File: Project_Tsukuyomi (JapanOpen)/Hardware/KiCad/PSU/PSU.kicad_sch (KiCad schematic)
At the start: 52 parts, among them J1 USB_C_Receptacle_USB2.0, J2 Conn_01x08_Socket, J3 Conn_01x08_Socket, J4 Conn_01x04_Socket, J5 Conn_01x02_Socket, J6 Conn_01x02_Socket, Q1 PMOS, SW1 SW_Push, SW2 SW_Push, U1 W25Q128JVS, U2 RP2040, U3 SFH617A-1, U4 AZ1084-5.0, Y1 Crystal_GND24

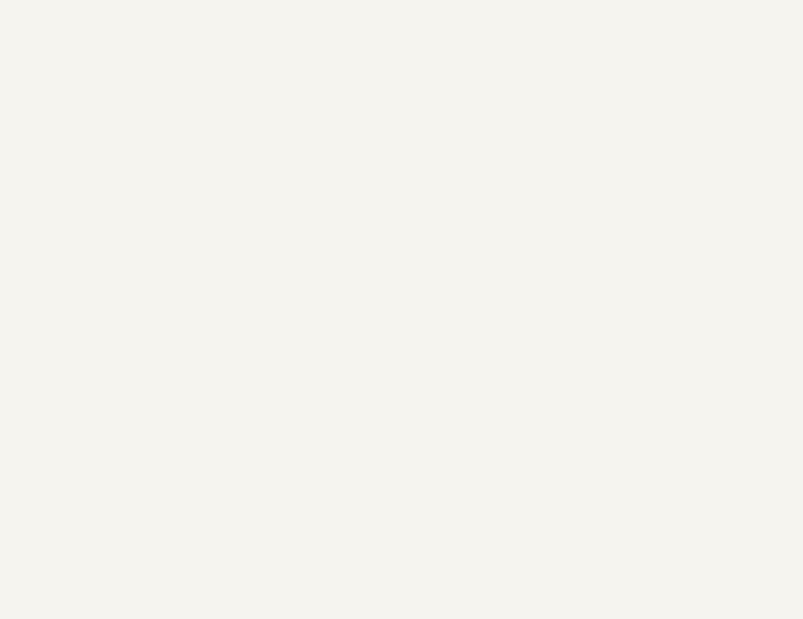
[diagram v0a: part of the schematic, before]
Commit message: KiCad変更
ごめんさい。溜めました
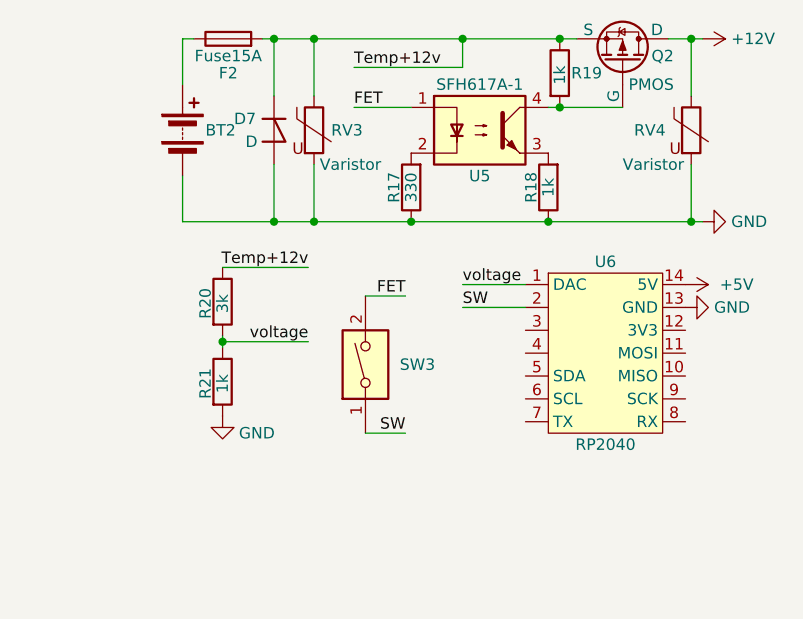
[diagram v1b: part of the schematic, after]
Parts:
- added BT2: Battery, Connector_AMASS:AMASS_XT60-M_1x02_P7.20mm_Vertical, symbol Device:Battery
- added D7: D, Diode_THT:D_DO-27_P12.70mm_Horizontal, symbol Device:D_Shockley
- added F2: Fuse15A, Fuse:Fuseholder_Clip-5x20mm_Littelfuse_520_Inline_P20.50x5.80mm_D1.30mm_Horizontal, symbol Device:Fuse
- added Q2: PMOS, Package_TO_SOT_SMD:TO-252-2, symbol Simulation_SPICE:PMOS
- added R17: 330, Resistor_SMD:R_0402_1005Metric, symbol Device:R
- added R18, R19, R21: 1k, Resistor_SMD:R_0402_1005Metric, symbol Device:R
- added R20: 3k, Resistor_SMD:R_0402_1005Metric, symbol Device:R
- added RV3, RV4: Varistor, Varistor:RV_Disc_D9mm_W3.3mm_P5mm, symbol Device:Varistor
- added SW3: SW_DIP_x01, symbol Switch:SW_DIP_x01
- added U5: SFH617A-1, Package_DIP:DIP-4_W7.62mm, symbol Isolator:SFH617A-1
- added U6: RP2040, symbol seeeduino_xiao:Seeeduino_Xiao
- C1, C11, C2, C3, C6, C7, C8, C9: LCSC (none) -> C1525
- C4, C5: LCSC (none) -> C1557
- R1, R15, R16, R2, R3, R4, R9: LCSC (none) -> C11702
- R10, R11: LCSC (none) -> C25905
- R12, R13: LCSC (none) -> C25100
- R14: LCSC (none) -> C25104
- R5: LCSC (none) -> C25076
- R8: LCSC (none) -> C25784
- U1: LCSC (none) -> C97521
- U2: LCSC (none) -> C2040
- Y1: LCSC (none) -> C7294610
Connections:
- net +12V: now also Q2.1 (D), RV4.1
- net FET: now also SW3.2, U5.1
- net GND: now also BT2.2 (-), D7.2 (A), R17.1, R18.1, R21.2, RV3.2, RV4.2, U6.13 (GND)
- net SW: now also SW3.1, U6.2
- net Temp+12v: now also D7.1 (K), F2.2, Q2.3 (S), R19.1, R20.1, RV3.1
- net voltage: now also R20.2, R21.1, U6.1 (DAC)
- new net: Q2.2 (G), R19.2, U5.4
- new net: BT2.1 (+), F2.1
- new net: R17.2, U5.2
- new net: R18.2, U5.3
- new net +5V: U6.14 (5V)
